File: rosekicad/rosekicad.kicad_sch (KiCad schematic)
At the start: 74 parts, among them J1 Solenoid, J10 Solenoid, J11 Solenoid, J12 Solenoid, J13 UV Lights, J14 LED Lights, J15 DMX Cable, J16 Barrel_Jack_MountingPin, J2 Solenoid, J3 Solenoid, J4 Solenoid, J5 Solenoid, J6 Solenoid, J7 Solenoid, J8 Solenoid, J9 Solenoid, Q1 2N2222, Q10 2N2222, Q11 2N2222, Q12 2N2222, Q13 2N2222, Q14 2N2222, Q15 2N2222, Q2 2N2222, Q3 2N2222, Q4 2N2222, Q5 2N2222, Q6 2N2222, Q7 2N2222, Q8 2N2222, Q9 2N2222, U1 MAX485E

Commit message: pcd built
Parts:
- D1: footprint Diode_THT:D_DO-35_SOD27_P10.16mm_Horizontal -> Diode_THT:D_DO-35_SOD27_P7.62mm_Horizontal
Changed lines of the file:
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@@
 			)
 		)
-		(property "Footprint" "Diode_THT:D_DO-35_SOD27_P10.16mm_Horizontal"
+		(property "Footprint" "Diode_THT:D_DO-35_SOD27_P7.62mm_Horizontal"
 			(at 95.25 68.58 0)
 			(effects

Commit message: added footprint
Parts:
- U1: footprint Package_SO:SOIC-8_3.9x4.9mm_P1.27mm -> (none)
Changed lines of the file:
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@@
 			)
 		)
-		(property "Footprint" "Package_SO:SOIC-8_3.9x4.9mm_P1.27mm"
+		(property "Footprint" ""
 			(at 234.95 124.46 0)
 			(effects

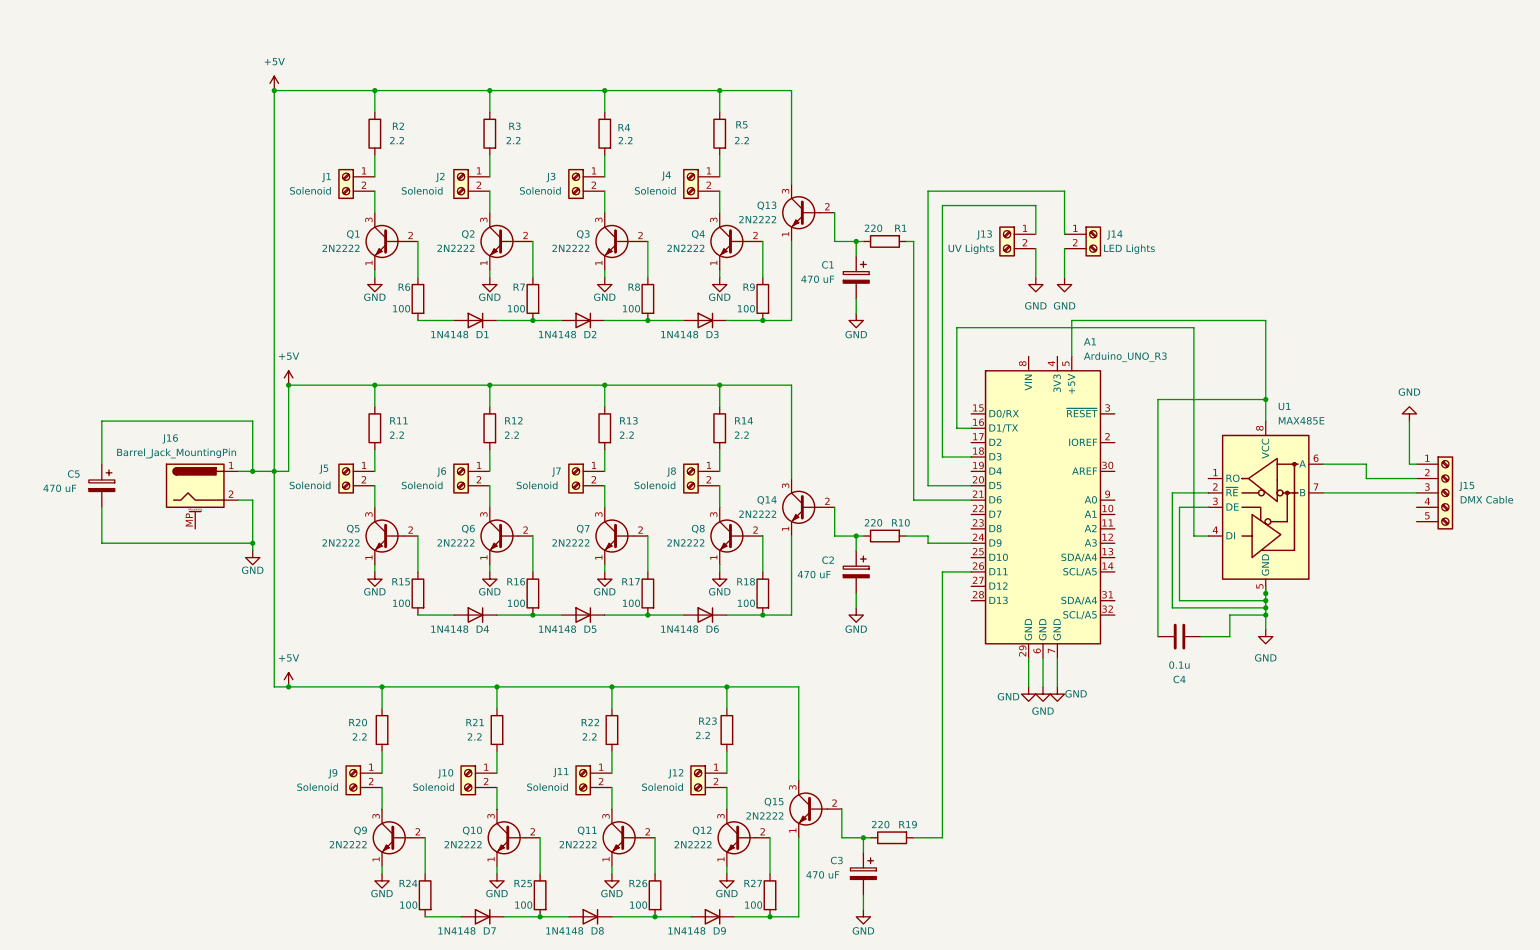
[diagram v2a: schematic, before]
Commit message: updated pcb
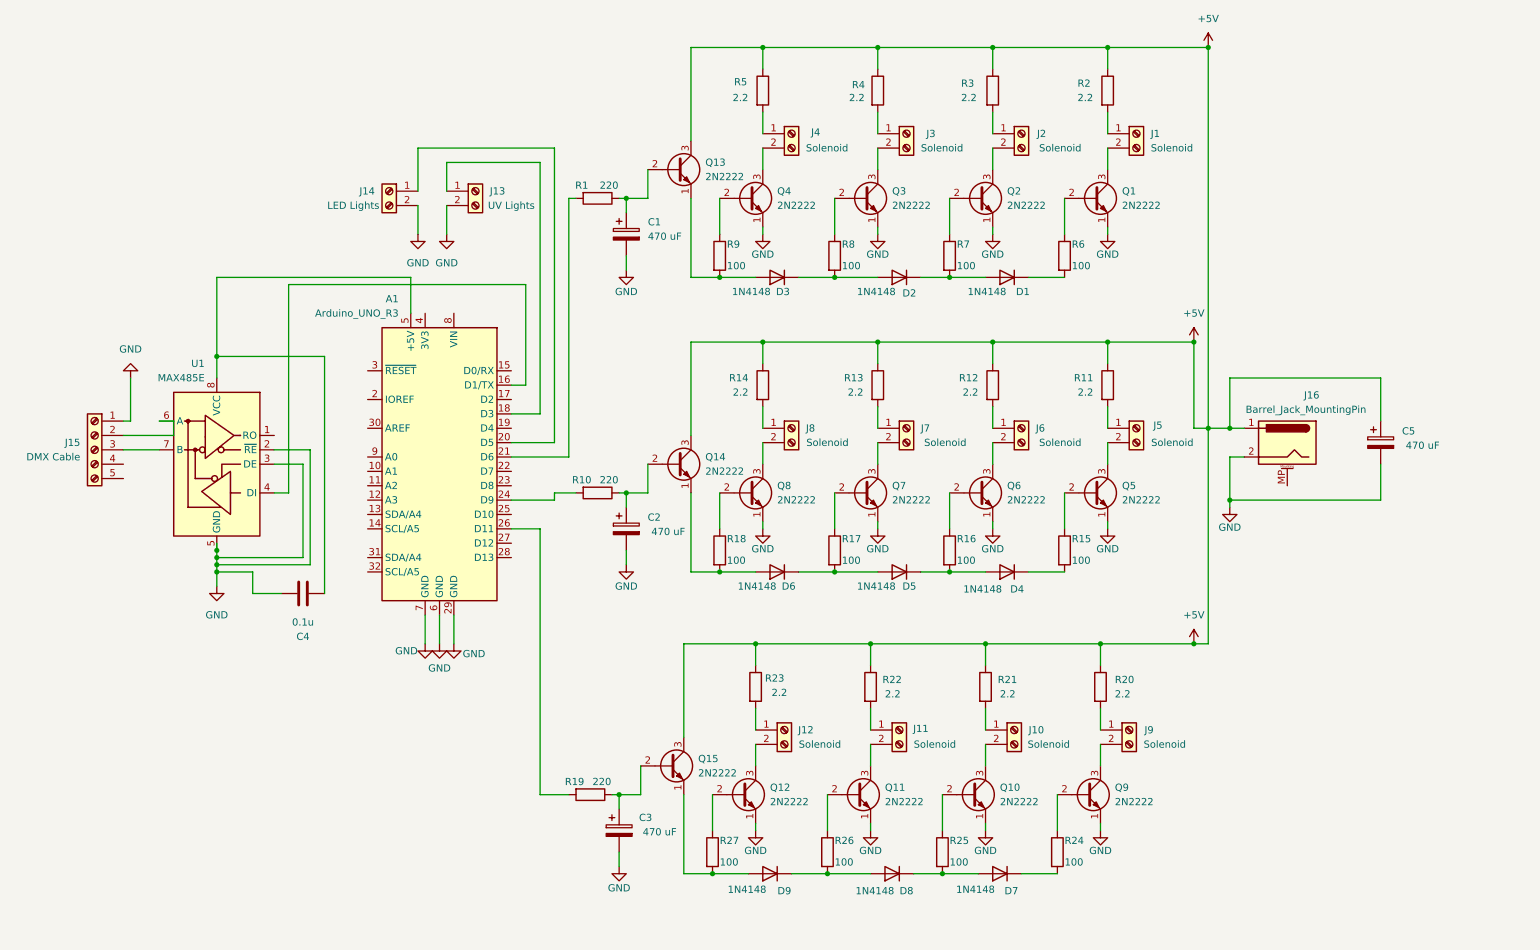
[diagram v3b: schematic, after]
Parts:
- U1: footprint (none) -> rosekicad:MAX485_Module
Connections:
- net at Q13.1 (E), R9.2: now also D3.2 (A); no longer D3.1 (K)
- net at Q15.1 (E), R27.2: now also D9.2 (A); no longer D9.1 (K)
- net at D4.2 (A): now also D5.1 (K), R16.2; no longer R15.2
- net at D7.2 (A): now also D8.1 (K), R25.2; no longer R24.2
- net at Q14.1 (E), R18.2: now also D6.2 (A); no longer D6.1 (K)
- net at D1.2 (A): now also D2.1 (K), R7.2; no longer R6.2
- new net: D8.2 (A), D9.1 (K), R26.2
- new net: D4.1 (K), R15.2
- new net: D5.2 (A), D6.1 (K), R17.2
- new net: D2.2 (A), D3.1 (K), R8.2
- new net: D7.1 (K), R24.2
- new net: D1.1 (K), R6.2
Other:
- moved on the sheet: A1, C1, C2, C3, C4, C5, D1, D2, D3, D4, D5, D6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
